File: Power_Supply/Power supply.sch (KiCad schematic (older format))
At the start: 54 parts, among them J1 Screw_Terminal_01x04, J2 Conn_01x04, K1 RY611012, Q1 BC548, U1 LM1084-12, U2 LM1084-5, U3 NE555P

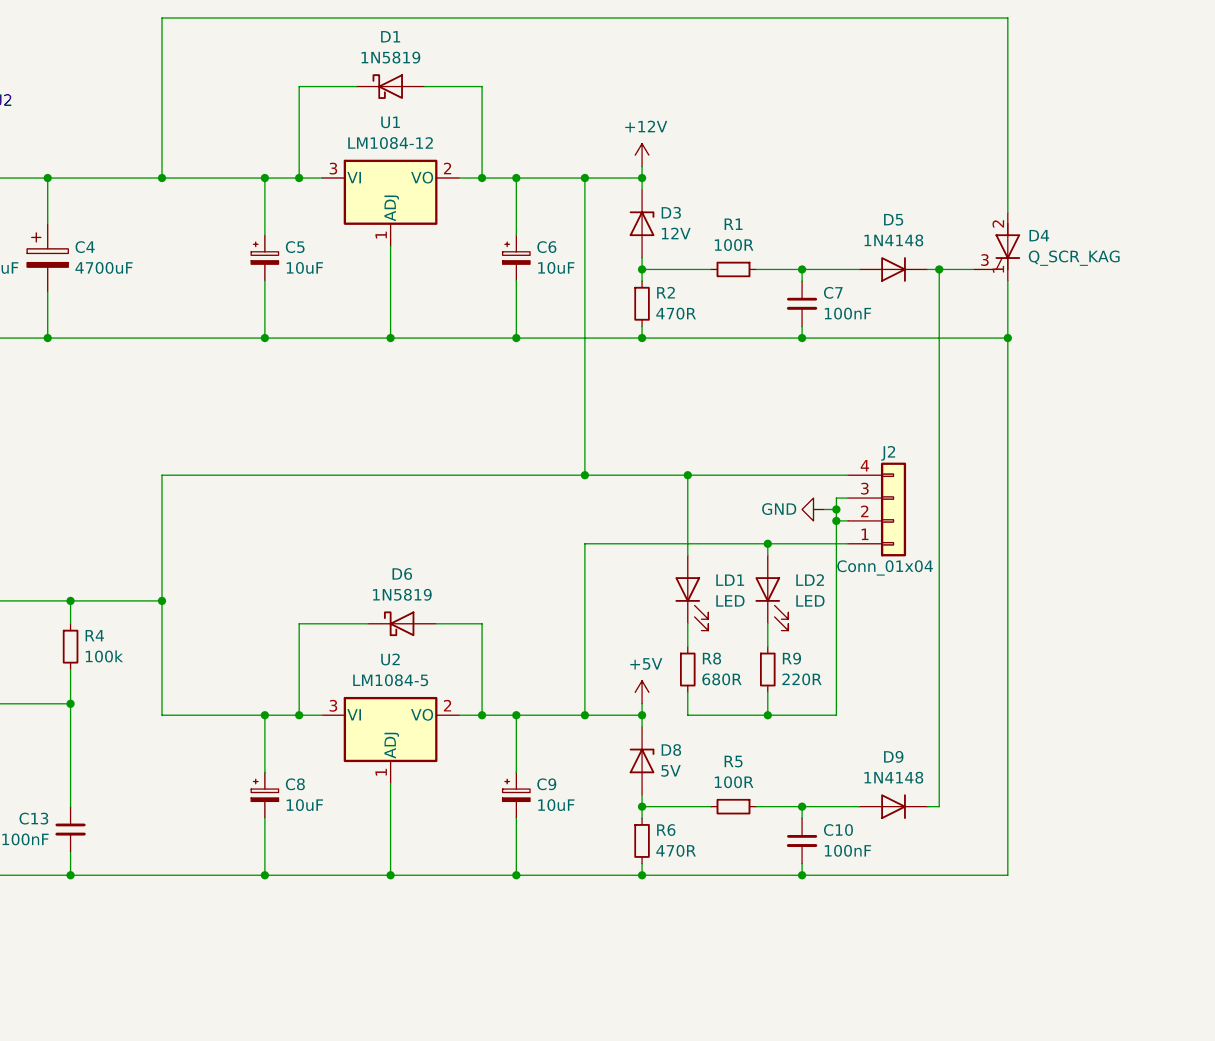
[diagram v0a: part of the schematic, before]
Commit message: PSU
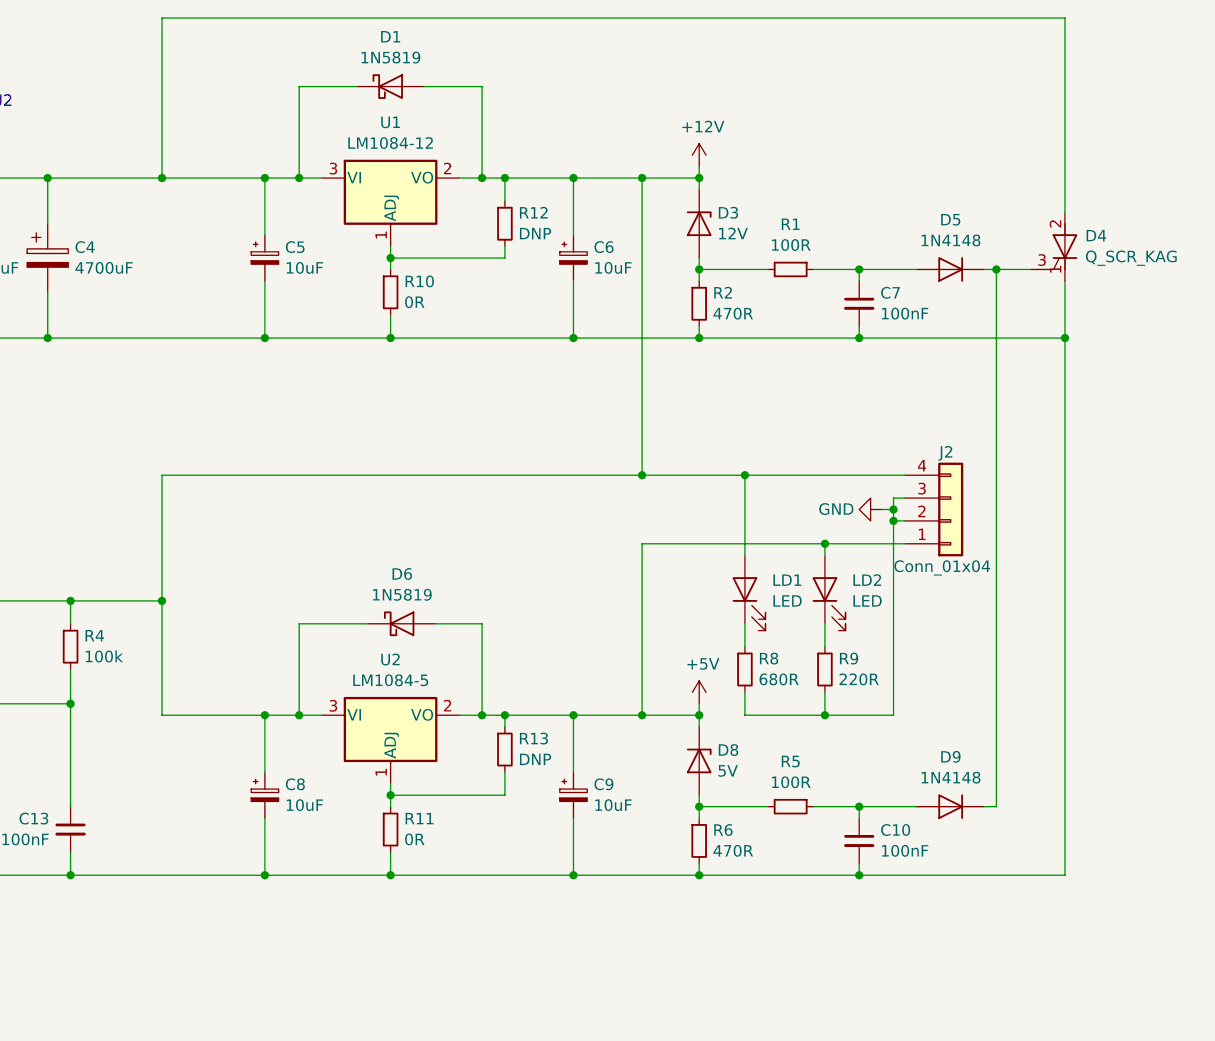
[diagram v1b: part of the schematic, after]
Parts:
- added R10, R11: 0R, Resistor_THT:R_Axial_DIN0207_L6.3mm_D2.5mm_P10.16mm_Horizontal, symbol Device:R_Small
- added R12, R13: DNP, Resistor_THT:R_Axial_DIN0207_L6.3mm_D2.5mm_P10.16mm_Horizontal, symbol Device:R_Small
- BR1: footprint Diode_THT:Diode_Bridge_Vishay_GBU -> ak:GBJ
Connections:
- net +12V: now also R12.1
- net +5V: now also R13.1
- net GND: now also R10.2, R11.2; no longer U1.1 (ADJ), U2.1 (ADJ)
- new net: R10.1, R12.2, U1.1 (ADJ)
- new net: R11.1, R13.2, U2.1 (ADJ)
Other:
- moved on the sheet: C10, C6, C7, C9, D3, D4, D5, D8, D9, J2, LD1, LD2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
